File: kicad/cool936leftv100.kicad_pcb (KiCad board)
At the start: 2 copper layers, 108.3 x 86.9 mm, 45 parts, among them J12 MJ-4PP-9, SW1 Switch_SW_Push, SW102 Switch_SW_Push, SW11 Switch_SW_Push, SW12 Switch_SW_Push, SW13 Switch_SW_Push, SW14 Switch_SW_Push, SW2 Switch_SW_Push, SW20 Switch_SW_Push, SW21 Switch_SW_Push, SW22 Switch_SW_Push, SW23 Switch_SW_Push, SW27 Switch_SW_Push, SW28 Switch_SW_Push, SW29 Switch_SW_Push, SW3 Switch_SW_Push, SW301 Switch_SW_Push, SW302 Switch_SW_Push, SW4 Switch_SW_Push, SW5 Switch_SW_Push, SW900 SW_PUSH, U1 ProMicro

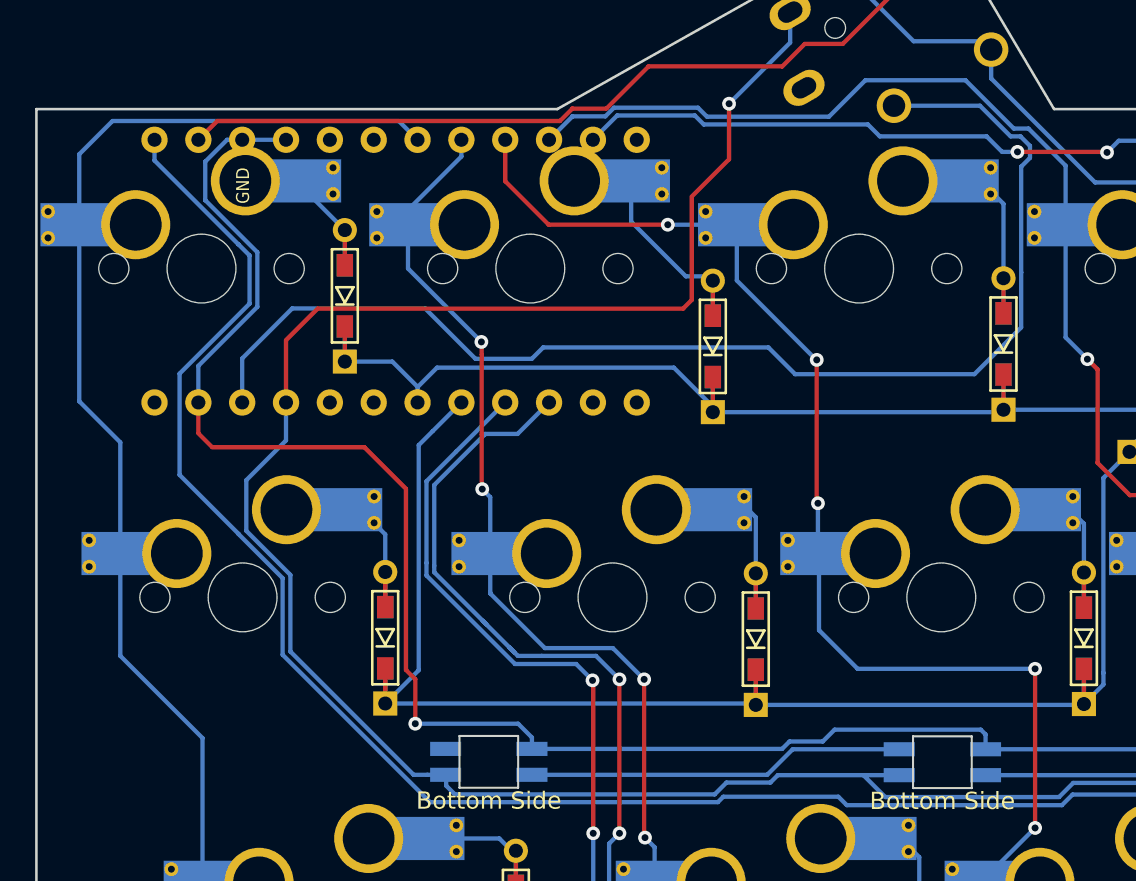
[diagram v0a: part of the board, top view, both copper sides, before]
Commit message: 修正
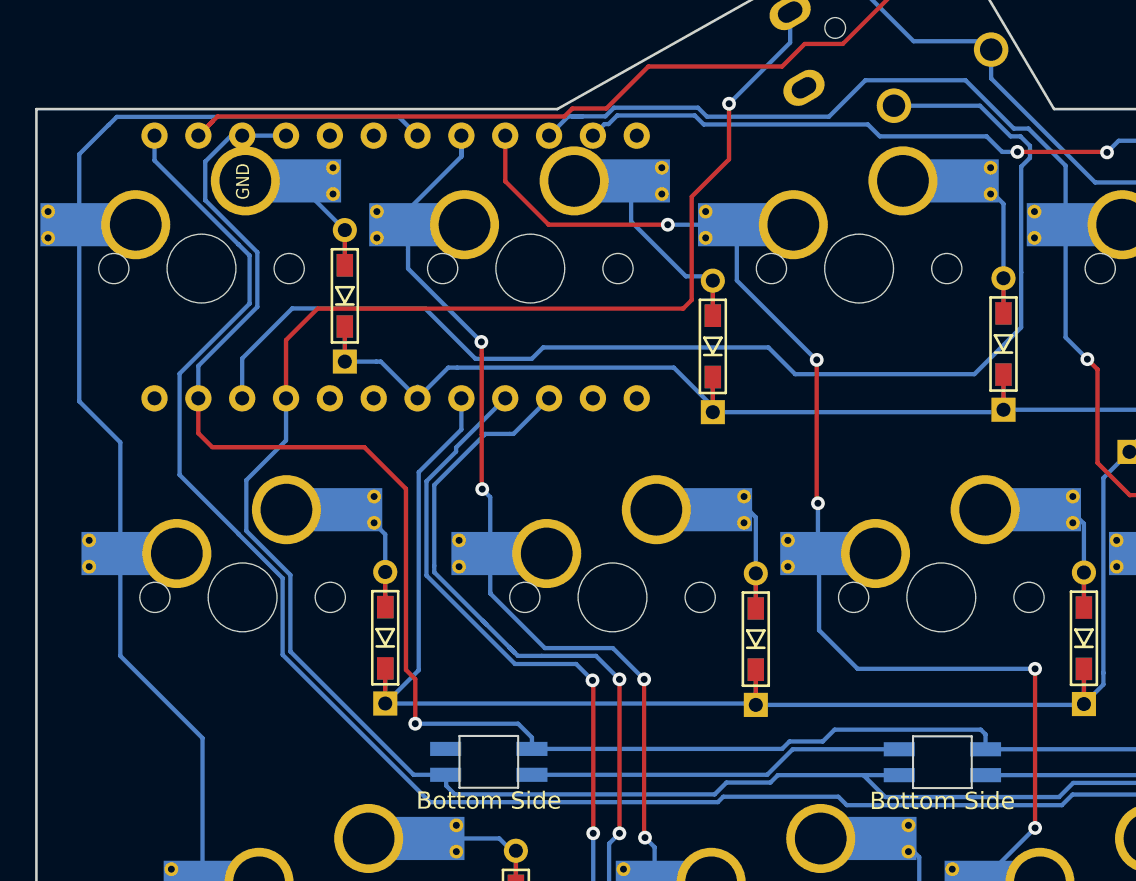
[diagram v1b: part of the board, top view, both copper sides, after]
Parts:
- moved U1 0.24 mm to (40.3, -0.09)
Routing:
- net col1L: track 85.3 -> 87.5 mm
- net DataL: track 46.2 -> 47.3 mm
- net row0L: track 83.3 -> 83.9 mm
- net col3L: track 123.3 -> 123.8 mm
